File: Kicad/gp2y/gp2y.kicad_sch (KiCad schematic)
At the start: 12 parts, among them K1 MOLEX-MICRO-LATCH-03-RIGHT-AN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, K2 MOLEX-MICRO-LATCH-04-RIGHT-AN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, U1 MCP1755-50

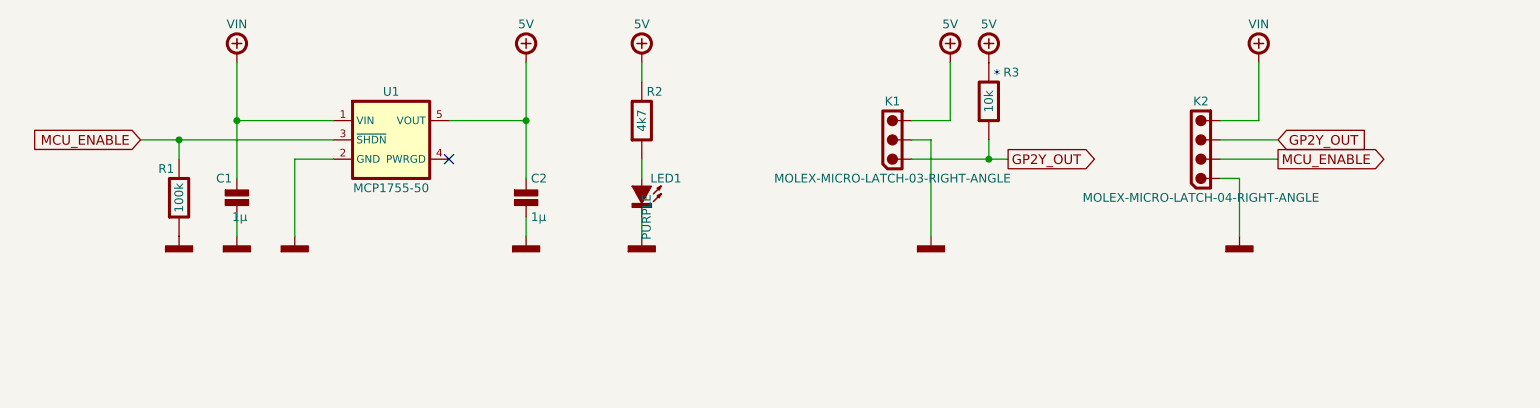
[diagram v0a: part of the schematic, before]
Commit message: Up
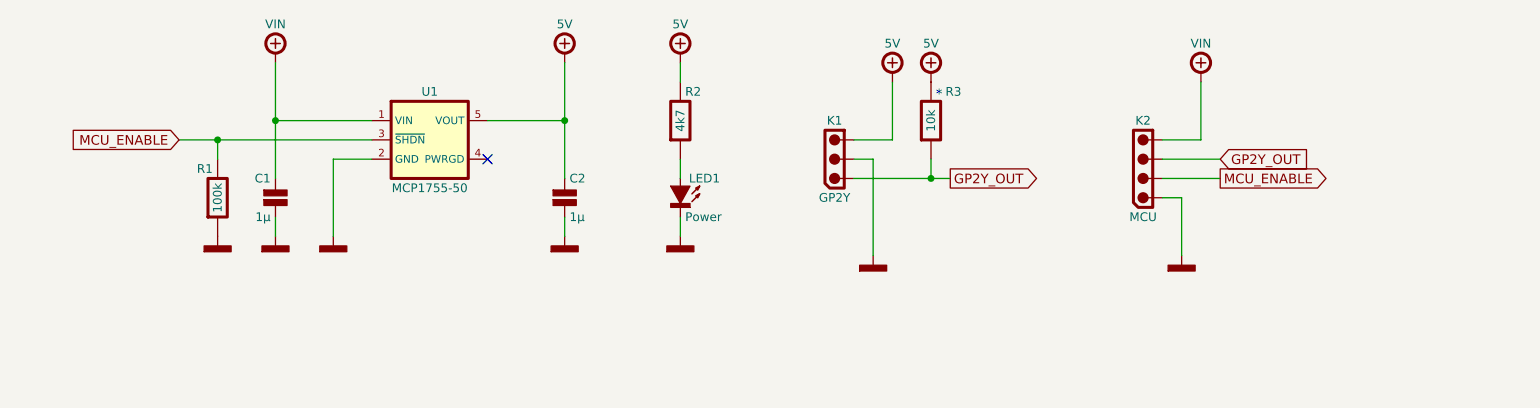
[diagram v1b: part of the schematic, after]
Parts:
- K1: value MOLEX-MICRO-LATCH-03-RIGHT-ANGLE -> GP2Y
- K2: value MOLEX-MICRO-LATCH-04-RIGHT-ANGLE -> MCU
- LED1: value PURPLE -> Power
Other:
- moved on the sheet: C1, C2, K1, K2, LED1, R1, R2, R3, U1
